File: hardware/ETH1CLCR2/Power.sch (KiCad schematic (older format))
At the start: 38 parts, among them Q901 IRFR5410, U901 NCS3S1205SC, U903 MAX5902, U905 NMK2409SAC, U907 NMK2409SC, U908 NCP1117-3.3_TO252, U909 NCP1117-5.0_TO252, U910 NCP1117-5.0_SOT223, U911 LT1175-5_SOT223

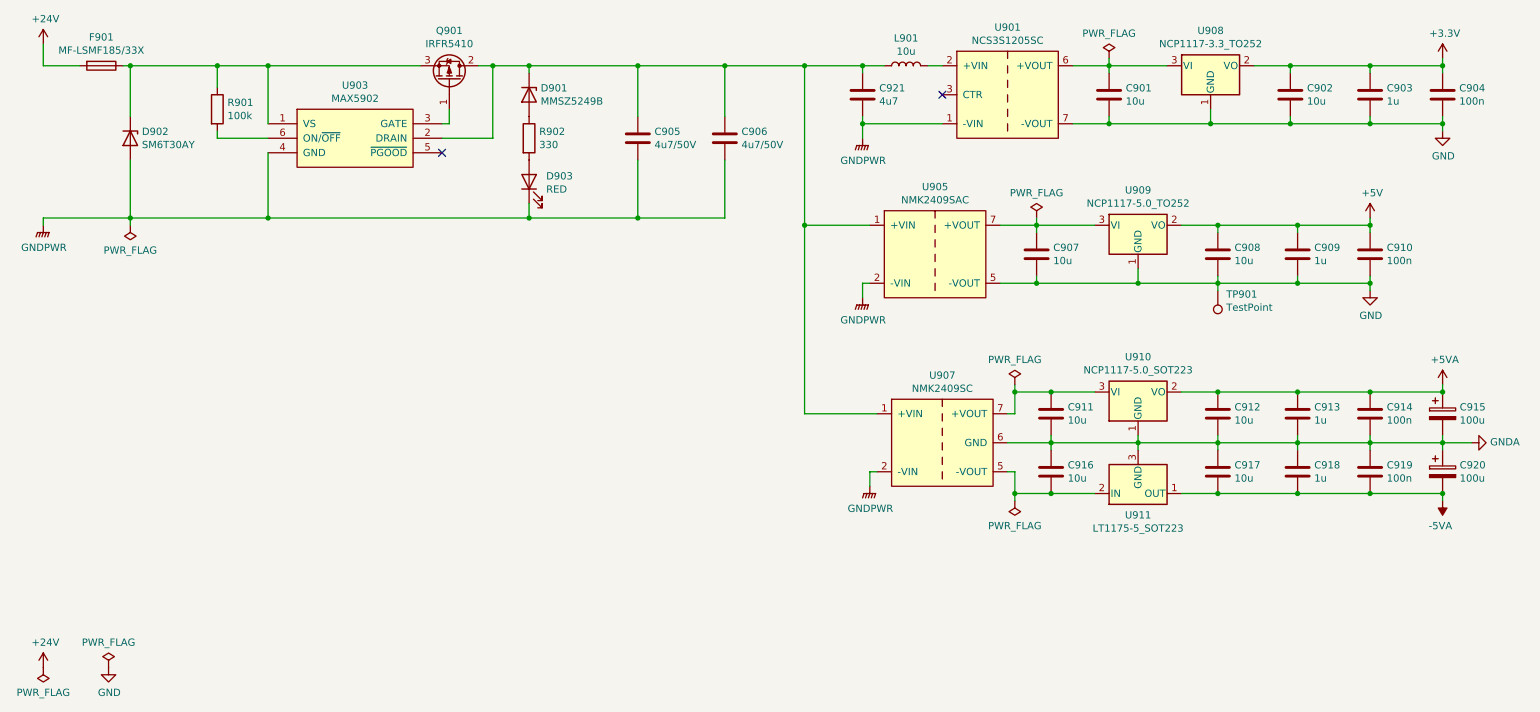
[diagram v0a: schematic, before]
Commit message: Footprints
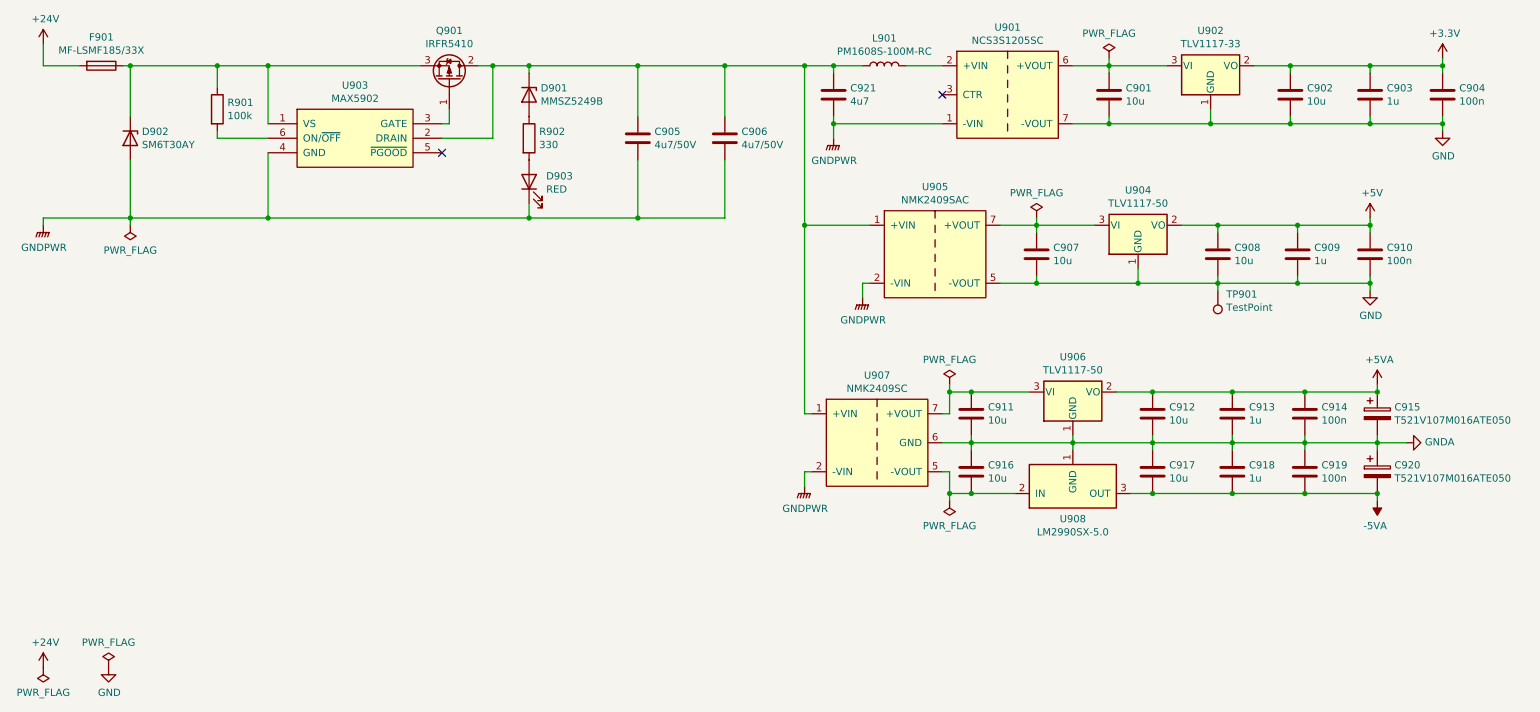
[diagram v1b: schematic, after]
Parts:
- removed U908: NCP1117-3.3_TO252, Package_TO_SOT_SMD:TO-252-2, symbol Regulator_Linear:NCP1117-3.3_TO252
- removed U909: NCP1117-5.0_TO252, Package_TO_SOT_SMD:TO-252-2, symbol Regulator_Linear:NCP1117-5.0_TO252
- removed U910: NCP1117-5.0_SOT223, Package_TO_SOT_SMD:SOT-223-3_TabPin2, symbol Regulator_Linear:NCP1117-5.0_SOT223
- removed U911: LT1175-5_SOT223, Package_TO_SOT_SMD:SOT-223-3_TabPin2, symbol Regulator_Linear:LT1175-5_SOT223
- added U902: TLV1117-33, Package_TO_SOT_SMD:TO-263-3_TabPin2, symbol Regulator_Linear:TLV1117-33
- added U904, U906: TLV1117-50, Package_TO_SOT_SMD:TO-263-3_TabPin2, symbol Regulator_Linear:TLV1117-50
- added U908: LM2990SX-5.0, Package_TO_SOT_SMD:TO-263-3_TabPin2, symbol Regulator_Linear:LM2990SX-5.0
- C915, C920: value 100u -> T521V107M016ATE050; footprint (none) -> Capacitor_Tantalum_SMD:CP_EIA-7343-20_Kemet-V_Pad2.25x2.55mm_HandSolder
- L901: value 10u -> PM1608S-100M-RC; footprint (none) -> ETH1CLCR2:PM1608S
- U901: footprint (none) -> ETH1CLCR2:NCS3
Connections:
- net +3V3: now also U902.2 (VO)
- net +5V: now also U904.2 (VO)
- net +5VA: now also U906.2 (VO)
- net -5VA: now also U908.3 (OUT)
- net GND: now also U902.1 (GND), U904.1 (GND)
- net GNDA: now also U906.1 (GND), U908.1 (GND)
- net at C907.1, U905.7 (+VOUT): now also U904.3 (VI)
- net at C916.2, U907.5 (-VOUT): now also U908.2 (IN)
- net at C911.1, U907.7 (+VOUT): now also U906.3 (VI)
- net at C901.1, U901.6 (+VOUT): now also U902.3 (VI)
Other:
- moved on the sheet: C911, C912, C913, C914, C915, C916, C917, C918, C919, C920, C921, L901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
